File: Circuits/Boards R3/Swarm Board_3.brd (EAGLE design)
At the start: 82.1 x 63.5 mm, 149 parts, among them CON1 ISP(2X3), CON2 MAIN_CONNECTOR_14, CON5 HEADER_3X1, CON7 MAIN_CONNECTOR_8, M1 VIBMOTOR, SW1 CL-SB-22A, T1 TEFT4300, T10 TEFT4300, T11 NPN2N2222, T12 SI2333DS-T1, T13 NPN2N2222, T14 NPN2N2222, T15 NPN2N2222, T16 NPN2N2222, T17 NPN2N2222, T18 NPN2N2222, T19 IRLML6244TR, T2 TEFT4300, T20 IRLML6244TR, T21 IRLML6244TR, T22 IRLML6244TR, T23 IRLML6244TR, T3 NPN2N2222, T4 TEFT4300, T5 TEFT4300, T6 TEFT4300, T7 TEFT4300, T8 TEFT4300, T9 TEFT4300, U2 MCP73833, U3 ATMEGA1281, U4 MCP9700A, U5 AH182, U6 AH182, U7 QRE1113, U8 QRE1113

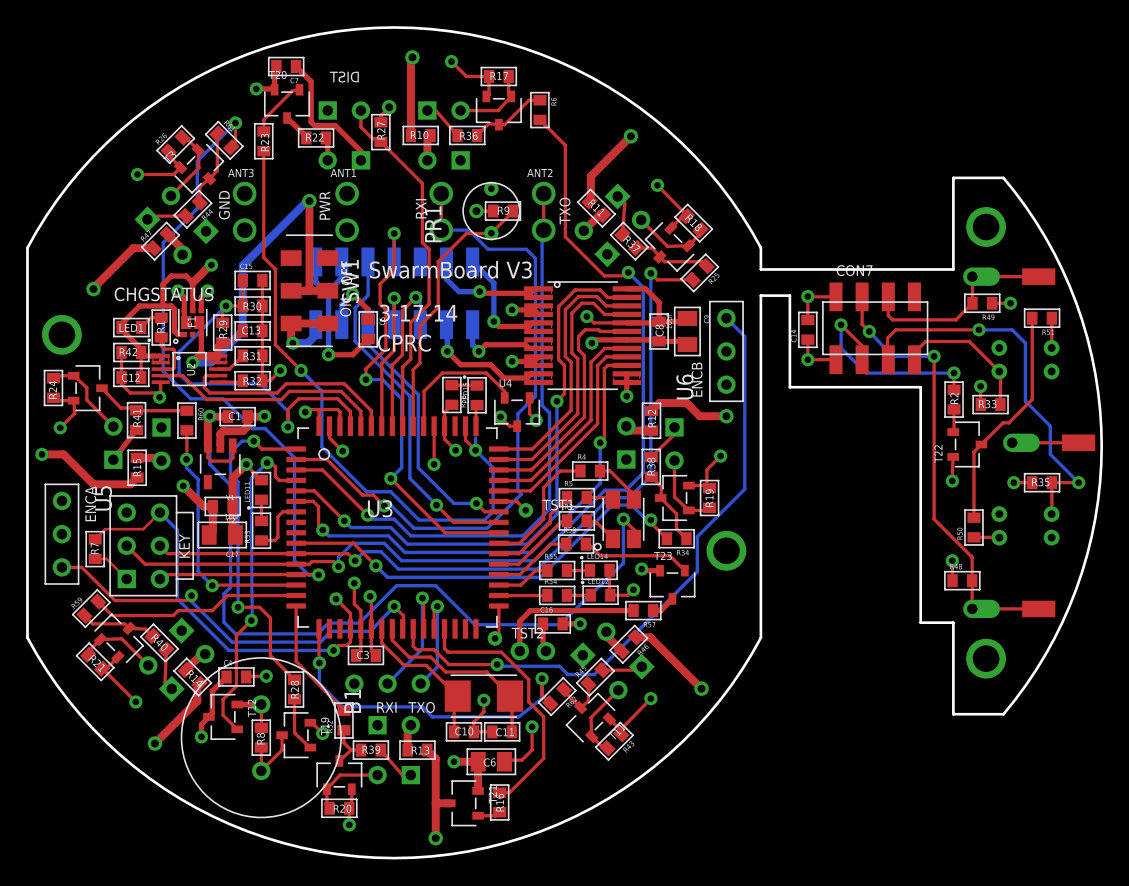
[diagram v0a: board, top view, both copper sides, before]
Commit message: Gerbers generated and zipped for boards and stencils
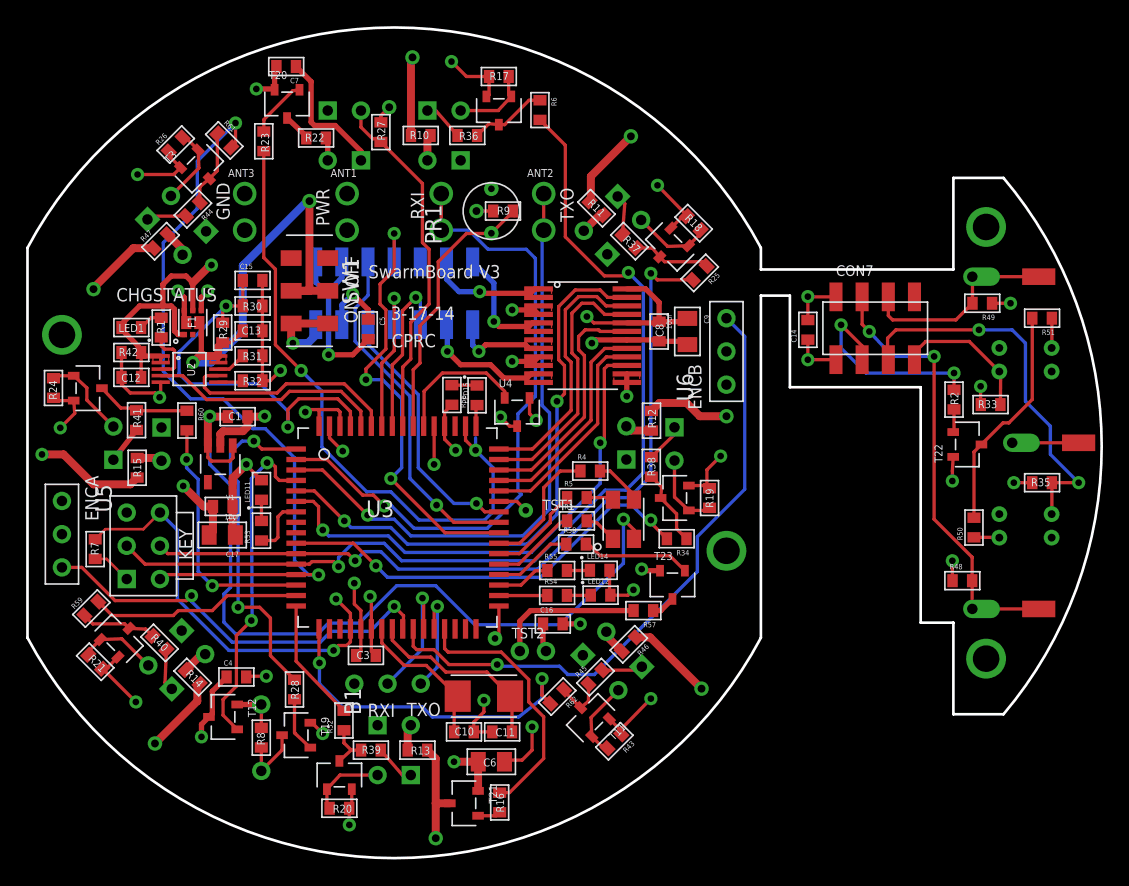
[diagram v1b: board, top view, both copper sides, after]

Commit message: BOMS and boards updated with a few slight value changes to reflect component availability
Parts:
- C3, C8: value .1uf -> 1uf
- R22: value 32 -> 30
- R3: value 200 -> 220
- R4, R5: value 70 -> 75
- XTAL1: value 10Mhz -> 8Mhz
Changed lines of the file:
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@@
 <attribute name="VALUE" x="18.713" y="32.4795" size="0.4064" layer="27"/>
 </element>
-<element name="C3" library="Passive" package="0603" value=".1uf" x="29.591" y="15.494" smashed="yes">
+<element name="C3" library="Passive" package="0603" value="1uf" x="29.591" y="15.494" smashed="yes">
 <attribute name="NAME" x="28.875" y="15.221" size="0.6096" layer="25"/>
 <attribute name="VALUE" x="28.521" y="14.224" size="0.4064" layer="27"/>
@@
 <attribute name="NAME" x="39.5605" y="7.62" size="0.6096" layer="25" rot="R180"/>
 </element>
-<element name="R22" library="Passive" package="0603" value="32" x="25.781" y="55.0545" smashed="yes">
+<element name="R22" library="Passive" package="0603" value="30" x="25.781" y="55.0545" smashed="yes">
 <attribute name="NAME" x="24.938" y="54.7815" size="0.6096" layer="25"/>
 <attribute name="VALUE" x="24.711" y="53.7845" size="0.4064" layer="27"/>
@@
 <attribute name="VALUE" x="6.973290625" y="34.870434375" size="0.4064" layer="27" rot="R90"/>
 </element>
-<element name="C8" library="Passive" package="0603" value=".1uf" x="52.0065" y="40.259" smashed="yes" rot="R270">
+<element name="C8" library="Passive" package="0603" value="1uf" x="52.0065" y="40.259" smashed="yes" rot="R270">
 <attribute name="NAME" x="51.7335" y="40.848" size="0.6096" layer="25" rot="R270"/>
 <attribute name="VALUE" x="50.7365" y="41.329" size="0.4064" layer="27" rot="R270"/>
@@
 <attribute name="VALUE" x="80.21" y="27.432" size="0.4064" layer="27"/>
 </element>
-<element name="XTAL1" library="Passive" package="SMDXTAL" value="10Mhz" x="38.608" y="12.3825" smashed="yes" rot="R180">
+<element name="XTAL1" library="Passive" package="SMDXTAL" value="8Mhz" x="38.608" y="12.3825" smashed="yes" rot="R180">
 <attribute name="VALUE" x="40.508" y="14.9825" size="0.6096" layer="27" rot="R180"/>
 </element>
@@
 <element name="B1" library="Passive" package="PIEZOBUZZER" value="PIEZOBUZZERPTH" x="21.59" y="9.2075" rot="R270"/>
 <element name="LED10" library="Passive" package="PLCC4" value="SMD_RGB" x="49.276" y="25.908" rot="R90"/>
-<element name="R3" library="Passive" package="0603" value="200" x="45.72" y="25.781"/>
-<element name="R4" library="Passive" package="0603" value="70" x="46.736" y="29.591"/>
-<element name="R5" library="Passive" package="0603" value="70" x="45.72" y="27.559"/>
+<element name="R3" library="Passive" package="0603" value="220" x="45.72" y="25.781"/>
+<element name="R4" library="Passive" package="0603" value="75" x="46.736" y="29.591"/>
+<element name="R5" library="Passive" package="0603" value="75" x="45.72" y="27.559"/>
 <element name="CON5" library="Mechanical" package="3PINHEADER_.100&quot;" value="HEADER_3X1" x="31.242" y="13.335" rot="MR0"/>
 <element name="U3" library="DigitalIC" package="TQFP64" value="ATMEGA1281" x="32.004" y="25.273"/>
